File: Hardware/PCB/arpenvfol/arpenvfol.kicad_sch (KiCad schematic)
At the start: 76 parts, among them J1 Synth_power_2x5, J10 3_pin_Molex_header, J11 2_pin_Molex_connector, J12 2_pin_Molex_header, J2 AudioJack2_SwitchT, J3 AudioJack2_SwitchT, J4 AudioJack2_SwitchT, J5 AudioJack2, J6 AudioJack2, J7 2_pin_Molex_connector, J8 2_pin_Molex_header, J9 3_pin_Molex_connector, Q1 BC549, Q2 BC549, U1 TL074

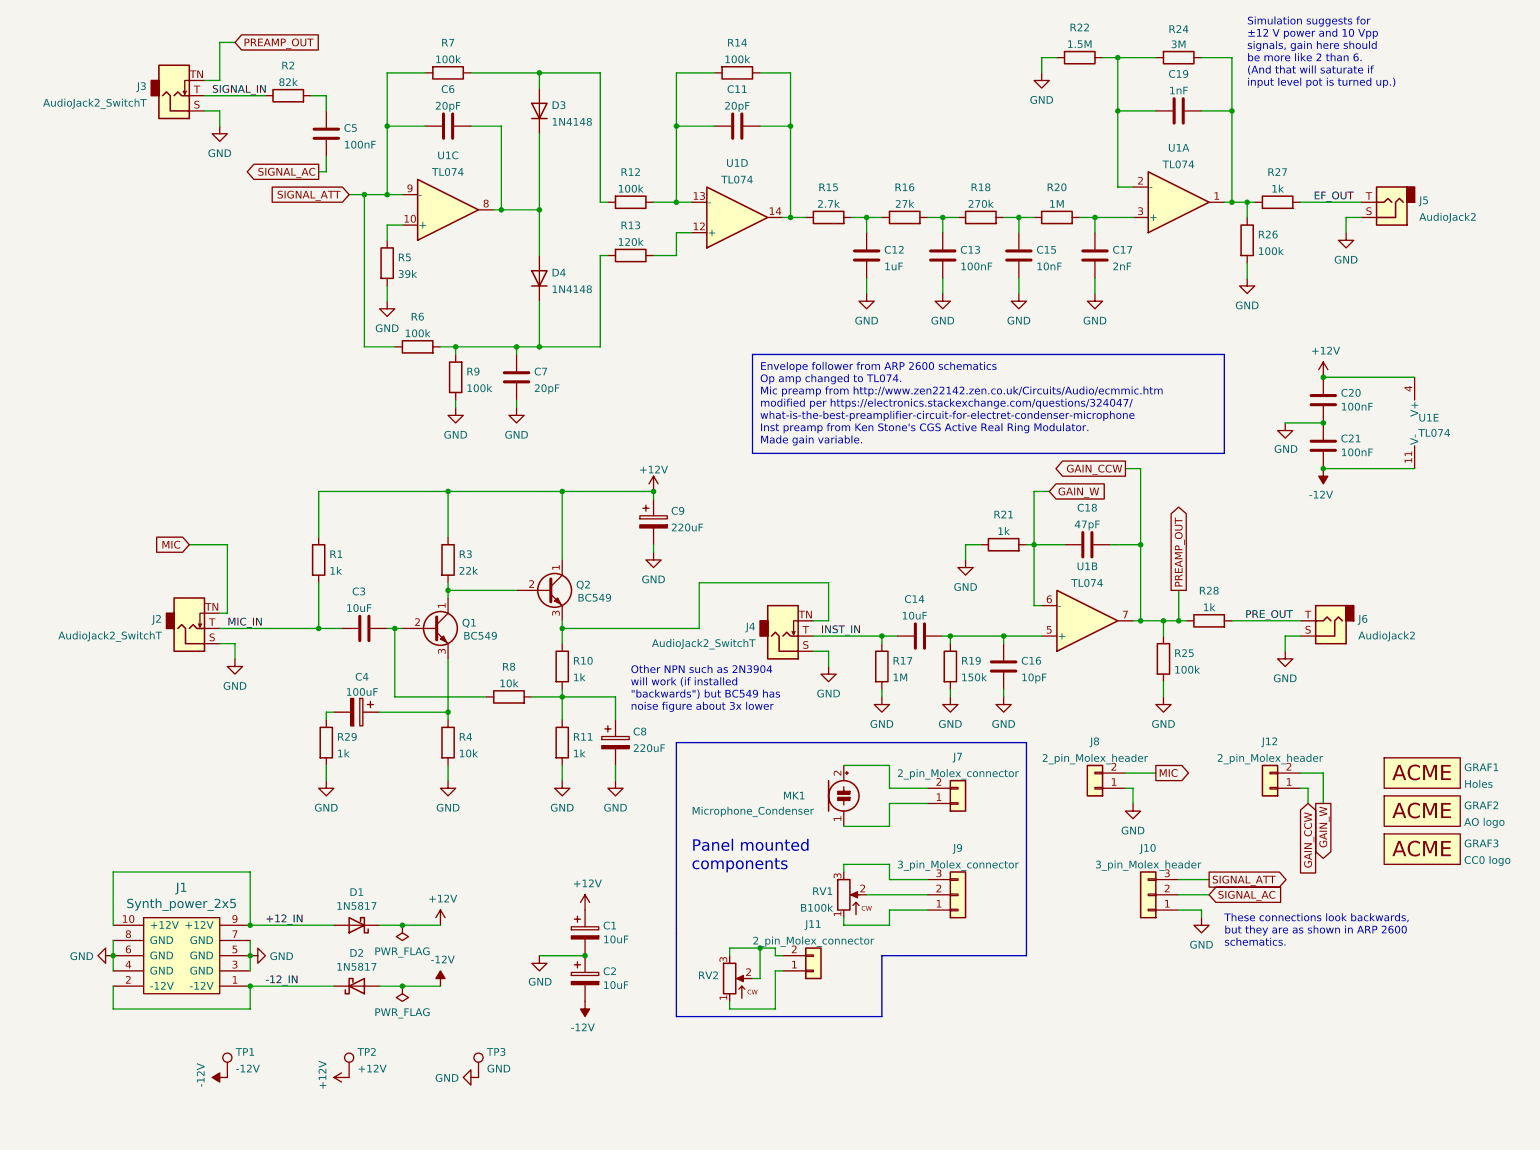
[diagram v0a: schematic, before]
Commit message: Schem reorg
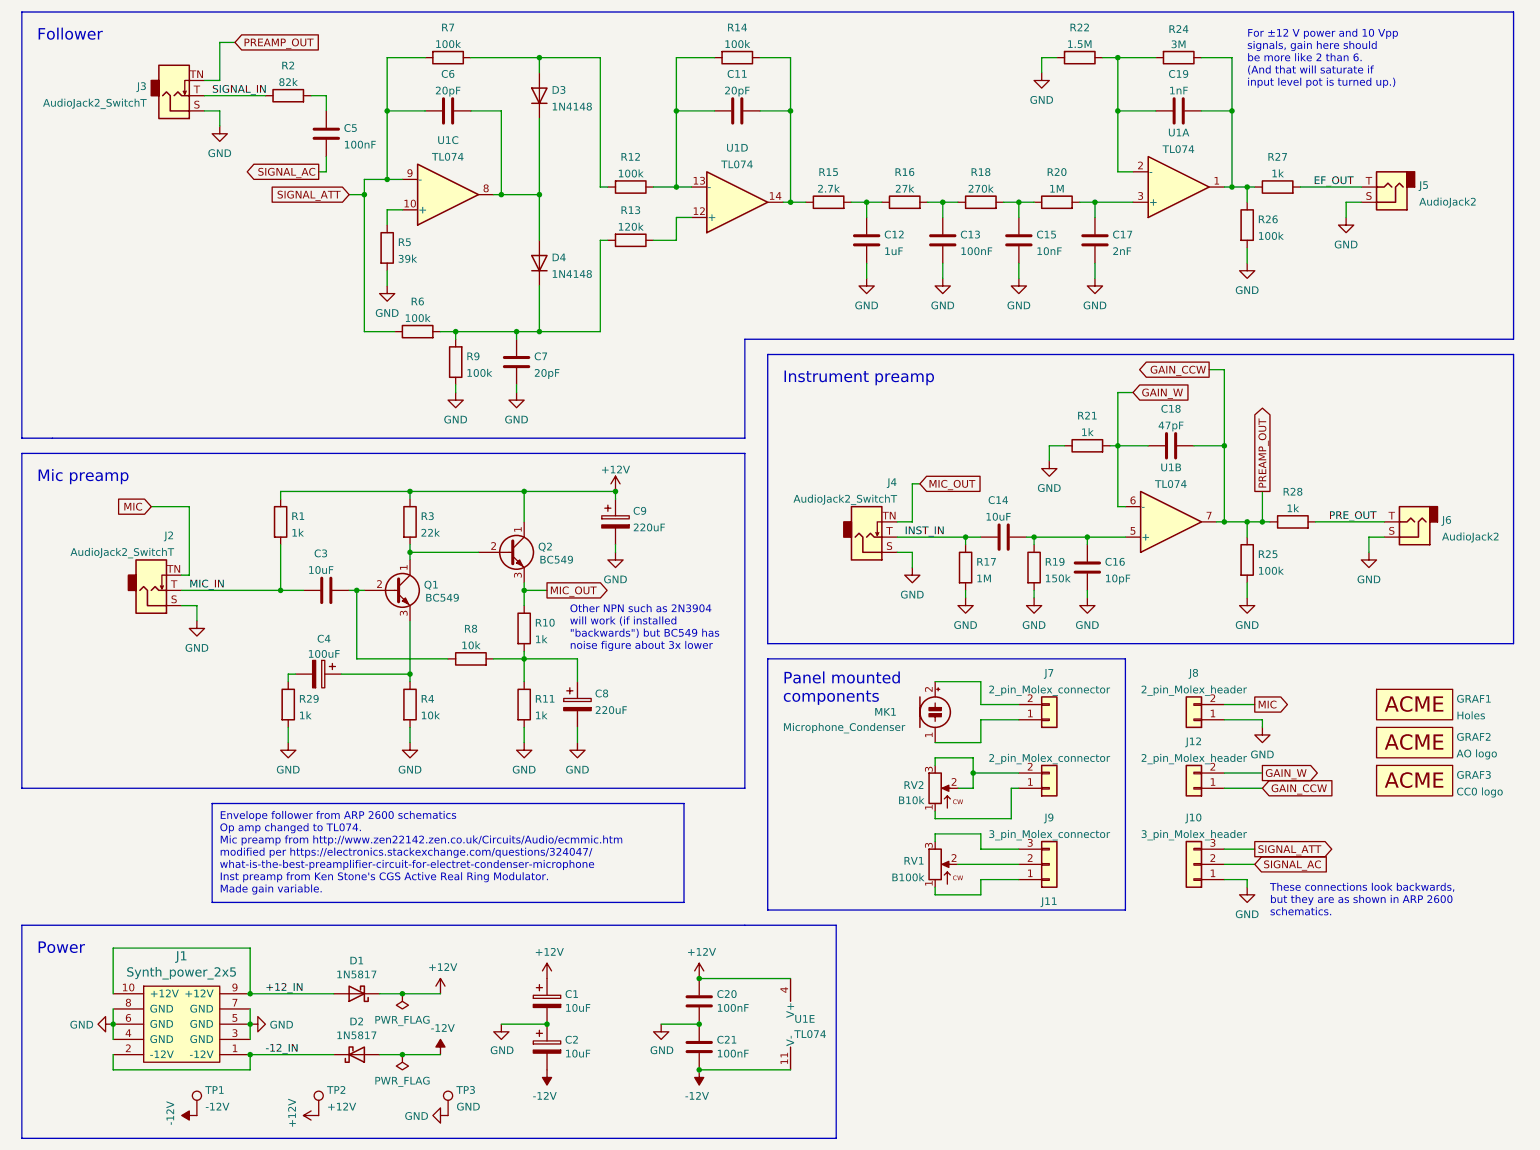
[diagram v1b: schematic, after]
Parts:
- C11, C16, C18, C6, C7: footprint (none) -> ao_tht:C_Disc_D5.0mm_W2.5mm_P5.00mm
- C12: footprint (none) -> ao_tht:C_Rect_L7.2mm_W7.2mm_P5.00mm_FKS2_FKP2_MKS2_MKP2
- C13, C15, C17, C19, C5: footprint (none) -> ao_tht:C_Rect_L7.2mm_W2.5mm_P5.00mm_FKS2_FKP2_MKS2_MKP2
- C14, C3: footprint (none) -> ao_tht:C_Radial_D8.0mm_H11.5mm_P3.50mm
- Q1, Q2: footprint (none) -> ao_tht:TO-92_Inline_Wide
- RV2: value (none) -> B10k
- TP3: footprint (none) -> ao_tht:TestPoint_THTPad_1.5x1.5mm_Drill0.7mm
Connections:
- net MIC_OUT: now reaches J4.TN, Q2.3 (E), R10.1
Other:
- note added: "Follower"
- note added: "For ±12 V power and 10 Vpp signals, gain here should be more like 2 than 6. (And that will saturate if input level pot is turned up.)"
- note added: "Instrument preamp"
- note added: "Mic preamp"
- note added: "Power"
- note removed: "Simulation suggests for ±12 V power and 10 Vpp signals, gain here should be more like 2 than 6. (And that will saturate if input level pot is turned up.)"
- moved on the sheet: C1, C11, C12, C13, C14, C15, C16, C17, C18, C2, C20, C21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
